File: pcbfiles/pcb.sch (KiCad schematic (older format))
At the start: 54 parts, among them J1 Conn_01x04_Female, Q1 AO3401A, SW1 SW_SPST, SW38 SW_SPDT, U2 XC6206, U3 TP4054, U4 nRF52840_holyiot_18010

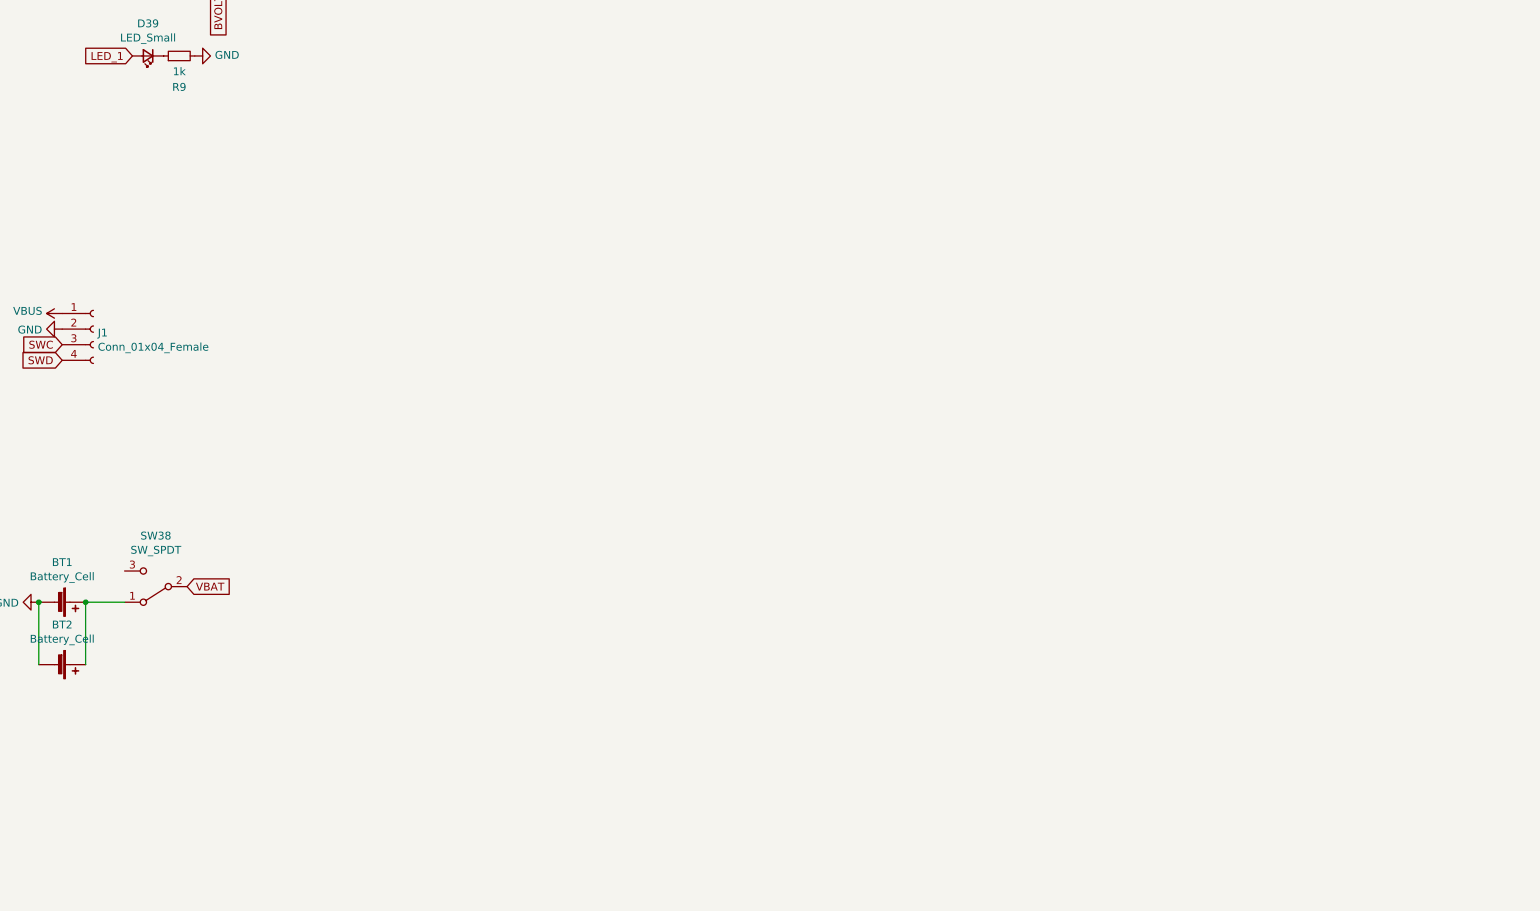
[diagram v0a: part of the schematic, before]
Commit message: continue schematic, test pcb idea
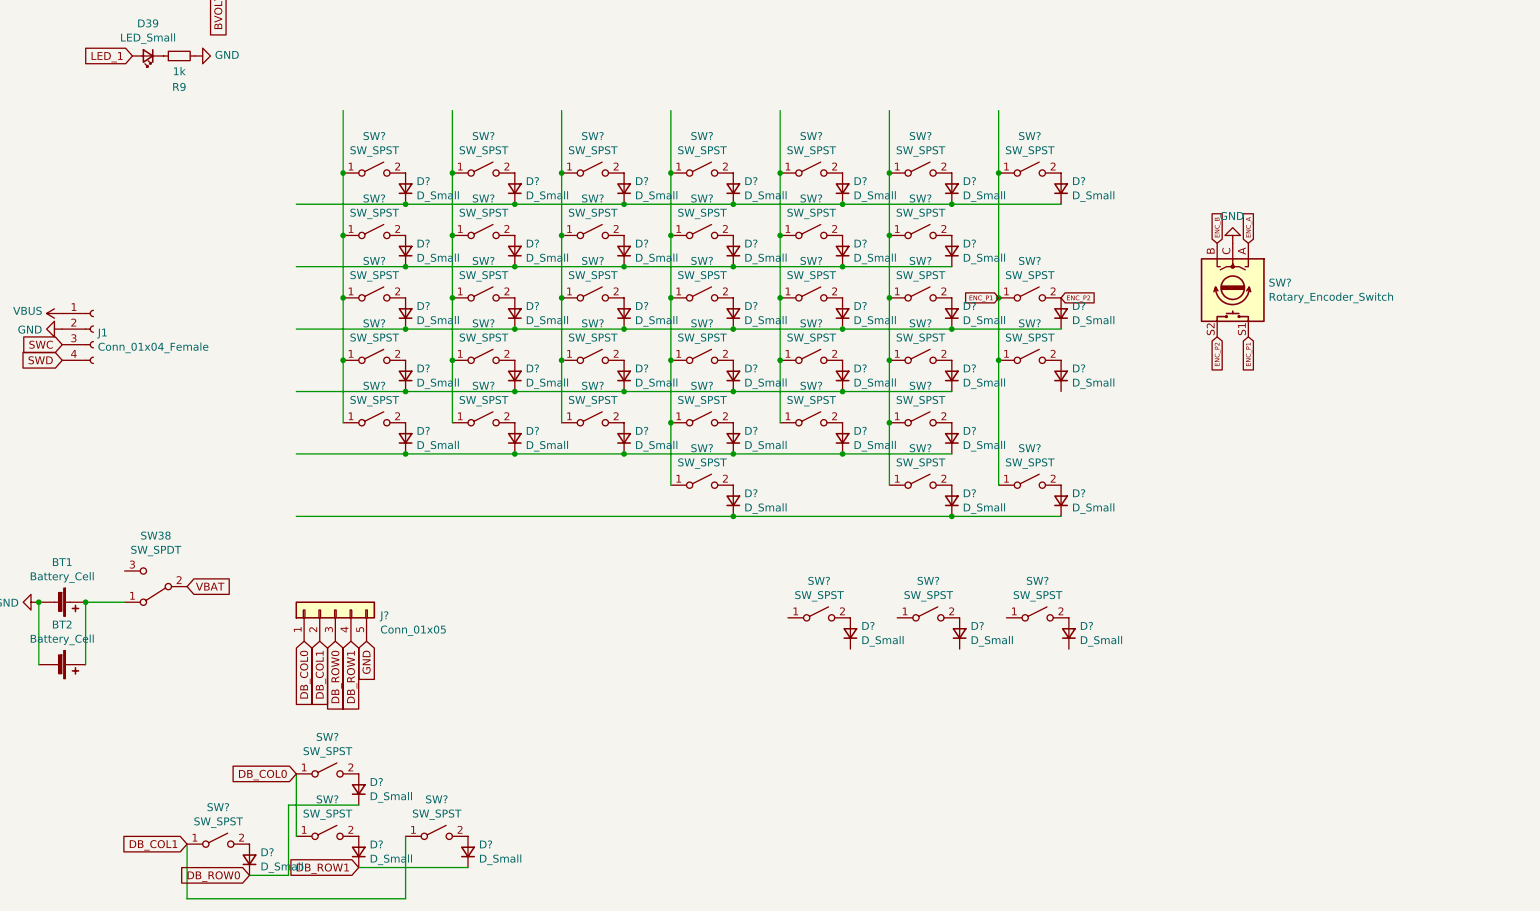
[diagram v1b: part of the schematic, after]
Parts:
- added D? (x43): D_Small, symbol Device:D_Small
- added J?: Conn_01x05, symbol Connector_Generic:Conn_01x05
- added SW? (x43): SW_SPST, symbol Switch:SW_SPST
- added SW?: Rotary_Encoder_Switch, symbol Device:Rotary_Encoder_Switch
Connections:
- net labels added: DB_COL0, DB_COL1, DB_ROW0, DB_ROW1, ENC_A, ENC_B, ENC_P1, ENC_P2
- wire segments 114 -> 193
